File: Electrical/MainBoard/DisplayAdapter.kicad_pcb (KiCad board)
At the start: 4 copper layers, 34 x 80 mm, 132 parts, among them J1 30_Pin_Zif, J2 4_Pin_Zif, J3 USB3_A, J4 USB_A, J5 USB_A, J6 Conn_ARM_SWD_TagConnect_TC203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, J7 2129691-2, M1 Standoff, M2 Standoff, M3 Standoff, M4 Standoff, M5 eDP-Adapter, Q1 PMOS, Q2 NPN, U1 STM32G0B1CETx, U2 MCP1665, U3 AP63357, U4 AP22653, U5 USB2514B, U6 TMUXHS4446, U7 INA234AxYBJ, U8 AP22653, U9 AP22653, Y1 24MHz

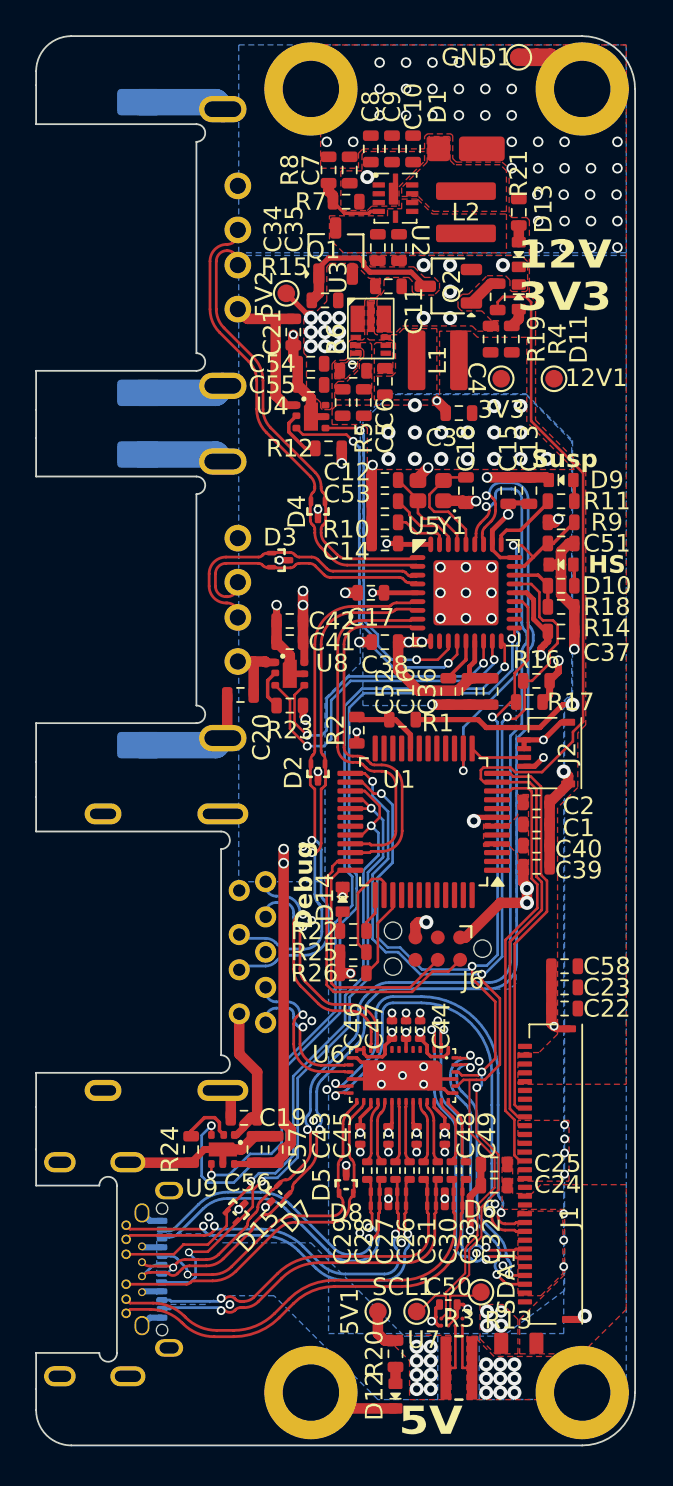
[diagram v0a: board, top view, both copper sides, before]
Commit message: Fixed Font issues
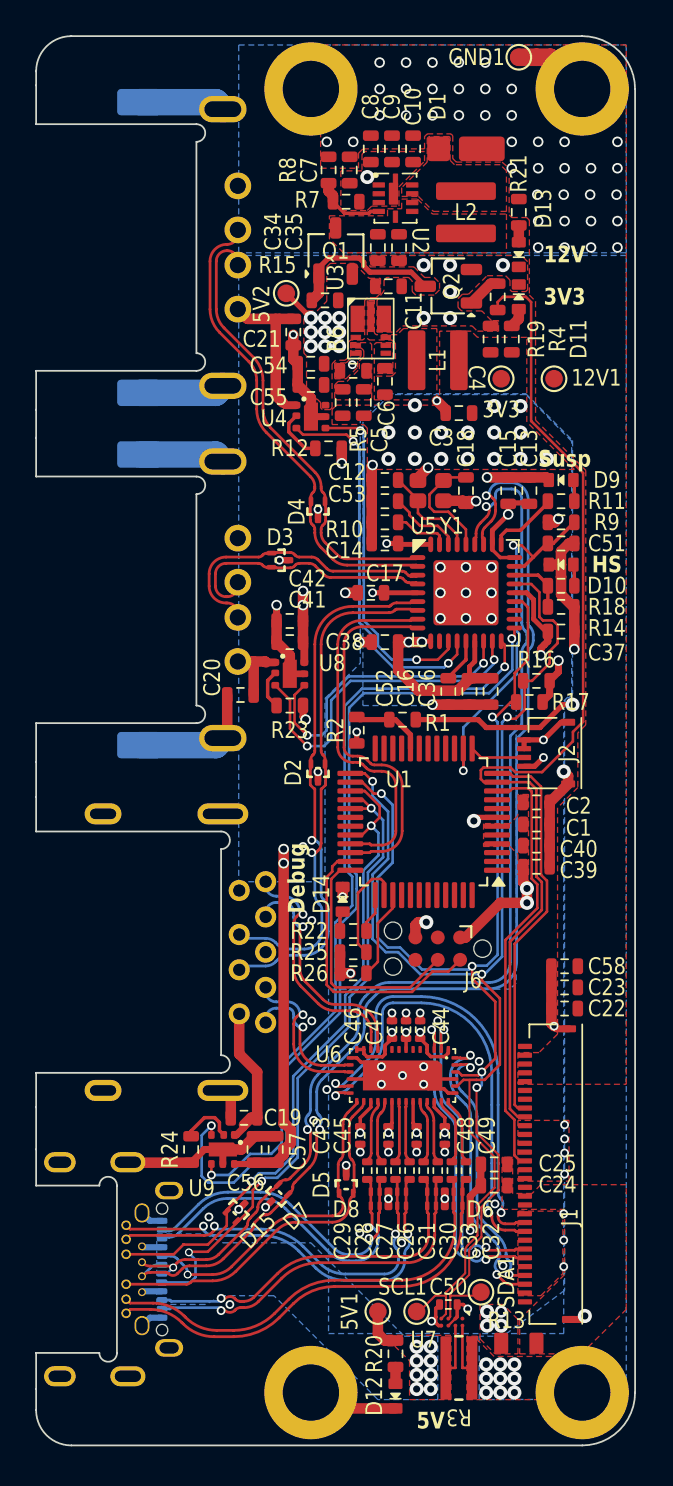
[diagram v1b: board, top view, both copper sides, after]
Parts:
- turned R3 to 180 degrees

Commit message: Added Mechanical components, fixed electrical err
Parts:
- C58: value 47u -> 22u
- R14, R9: value 36K -> 30K
- R15: value 10K -> 4K7
- R16, R17: value 1.2K -> 4K7
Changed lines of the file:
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@@
 			)
 		)
-		(property "Value" "36K"
+		(property "Value" "30K"
 			(at 8.95 4.4 180)
 			(unlocked yes)
@@
 			)
 		)
-		(property "Value" "47u"
+		(property "Value" "22u"
 			(at 8.95 4.4 0)
 			(unlocked yes)
@@
 			)
 		)
-		(property "Value" "1.2K"
+		(property "Value" "4K7"
 			(at 8.95 4.4 0)
 			(unlocked yes)
@@
 			)
 		)
-		(property "Value" "1.2K"
+		(property "Value" "4K7"
 			(at 8.95 4.4 0)
 			(unlocked yes)
@@
 			)
 		)
-		(property "Value" "36K"
+		(property "Value" "30K"
 			(at 8.95 4.4 180)
 			(unlocked yes)
@@
 			)
 		)
-		(property "Value" "10K"
+		(property "Value" "4K7"
 			(at 8.95 4.4 180)
 			(unlocked yes)
